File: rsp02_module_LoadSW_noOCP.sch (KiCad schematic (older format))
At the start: 9 parts, among them Q22 SISS23DN-T1-GE3, Q23 IRF7404, Q24 BC848B

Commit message: Update PCB
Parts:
- R90, R91, R92, R93: footprint Resistor_SMD:R_0402_1005Metric -> Resistor_SMD:R_0603_1608Metric
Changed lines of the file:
@@
 F 0 "R90" H 7000 1750 50  0000 L CNN
 F 1 "100k" H 7000 1550 50  0000 L CNN
-F 2 "Resistor_SMD:R_0402_1005Metric" V 6880 1650 50  0001 C CNN
+F 2 "Resistor_SMD:R_0603_1608Metric" V 6880 1650 50  0001 C CNN
 F 3 "~" H 6950 1650 50  0001 C CNN
 	1    6950 1650
@@
 F 0 "R93" H 9300 2250 50  0000 L CNN
 F 1 "100k" H 9300 2050 50  0000 L CNN
-F 2 "Resistor_SMD:R_0402_1005Metric" V 9180 2150 50  0001 C CNN
+F 2 "Resistor_SMD:R_0603_1608Metric" V 9180 2150 50  0001 C CNN
 F 3 "~" H 9250 2150 50  0001 C CNN
 	1    9250 2150
@@
 F 0 "R92" H 8850 5000 50  0000 L CNN
 F 1 "10k" H 8850 4800 50  0000 L CNN
-F 2 "Resistor_SMD:R_0402_1005Metric" V 8730 4900 50  0001 C CNN
+F 2 "Resistor_SMD:R_0603_1608Metric" V 8730 4900 50  0001 C CNN
 F 3 "~" H 8800 4900 50  0001 C CNN
 	1    8800 4900
@@
 F 0 "R91" V 8600 4550 50  0000 L CNN
 F 1 "10k" V 8400 4550 50  0000 L CNN
-F 2 "Resistor_SMD:R_0402_1005Metric" V 8430 4600 50  0001 C CNN
+F 2 "Resistor_SMD:R_0603_1608Metric" V 8430 4600 50  0001 C CNN
 F 3 "~" H 8500 4600 50  0001 C CNN
 	1    8500 4600

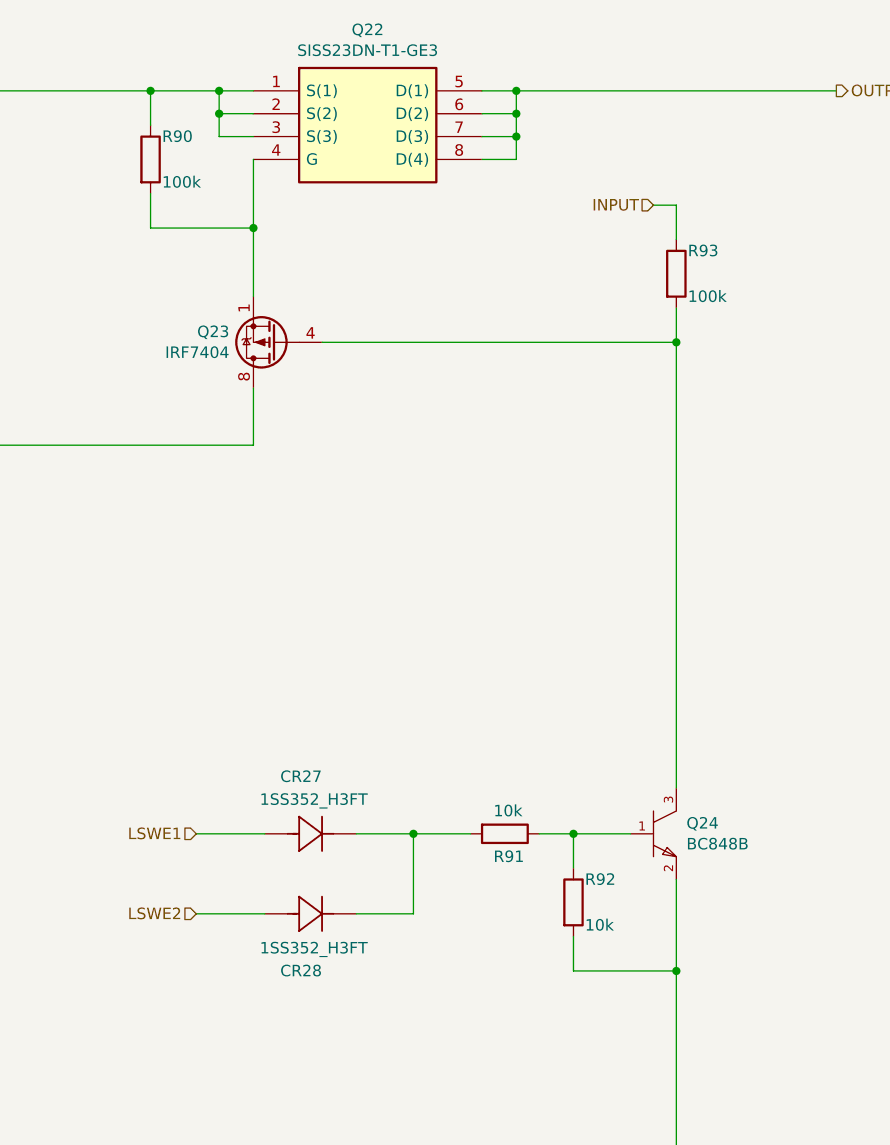
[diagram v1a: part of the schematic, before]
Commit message: PCB Update
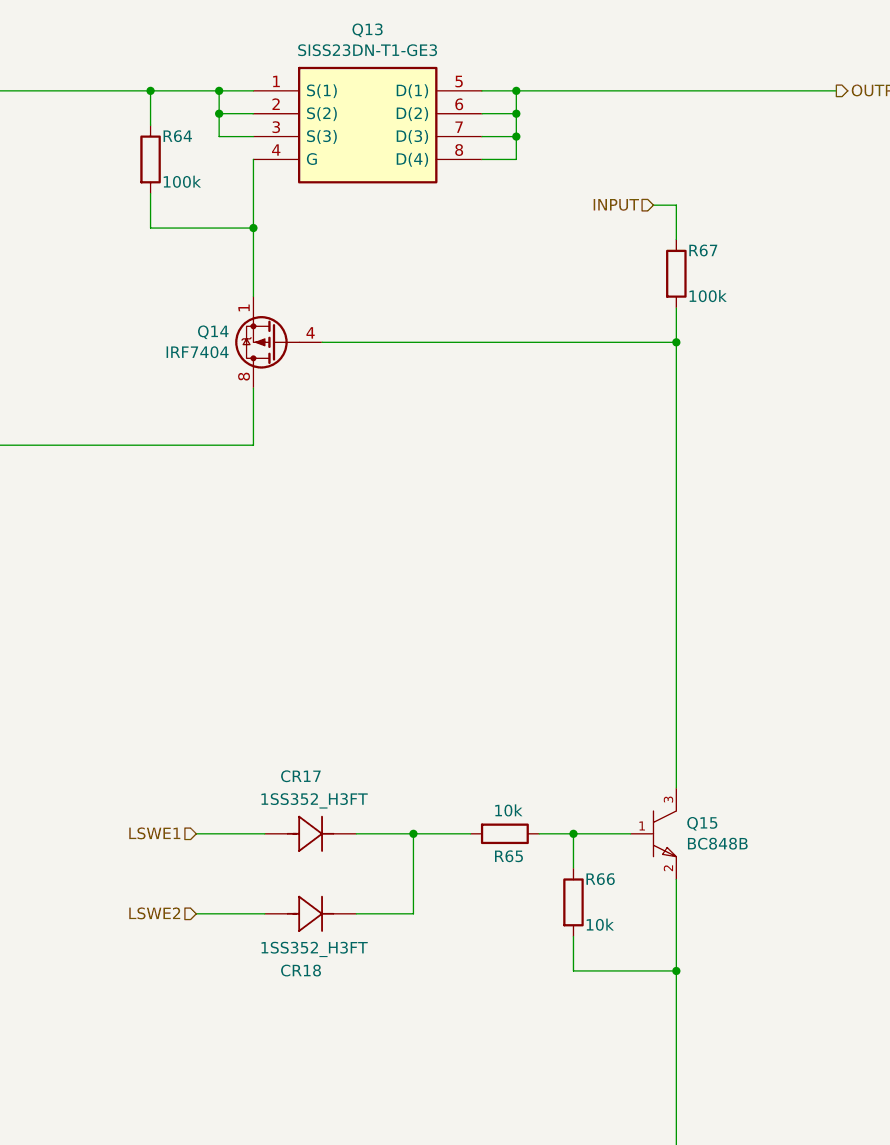
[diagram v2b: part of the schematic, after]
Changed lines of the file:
@@
 $Descr A4 11693 8268
 encoding utf-8
-Sheet 9 17
+Sheet 6 17
 Title "rsp02_module_LoadSW_OCP_noOCP"
 Date "2020-12-07"
@@
 AR Path="/5FD193EF/5FD0BC5C" Ref="Q22"  Part="1"
 AR Path="/5FD18D34/5FD0BC5C" Ref="Q13"  Part="1"
-F 0 "Q22" H 7900 1617 50  0000 C CNN
+F 0 "Q13" H 7900 1617 50  0000 C CNN
 F 1 "SISS23DN-T1-GE3" H 7900 1526 50  0000 C CNN
 F 2 "mypartsLib:POWERPAK-1212-8" H 7900 800 50  0001 C CNN
@@
 AR Path="/5FD193EF/5FD0BC5D" Ref="R90"  Part="1"
 AR Path="/5FD18D34/5FD0BC5D" Ref="R64"  Part="1"
-F 0 "R90" H 7000 1750 50  0000 L CNN
+F 0 "R64" H 7000 1750 50  0000 L CNN
 F 1 "100k" H 7000 1550 50  0000 L CNN
 F 2 "Resistor_SMD:R_0603_1608Metric" V 6880 1650 50  0001 C CNN
@@
 AR Path="/5FD193EF/5FD0BC5E" Ref="R93"  Part="1"
 AR Path="/5FD18D34/5FD0BC5E" Ref="R67"  Part="1"
-F 0 "R93" H 9300 2250 50  0000 L CNN
+F 0 "R67" H 9300 2250 50  0000 L CNN
 F 1 "100k" H 9300 2050 50  0000 L CNN
 F 2 "Resistor_SMD:R_0603_1608Metric" V 9180 2150 50  0001 C CNN
@@
 AR Path="/5FD193EF/5FD0BC5F" Ref="R92"  Part="1"
 AR Path="/5FD18D34/5FD0BC5F" Ref="R66"  Part="1"
-F 0 "R92" H 8850 5000 50  0000 L CNN
+F 0 "R66" H 8850 5000 50  0000 L CNN
 F 1 "10k" H 8850 4800 50  0000 L CNN
 F 2 "Resistor_SMD:R_0603_1608Metric" V 8730 4900 50  0001 C CNN
@@
 AR Path="/5FD193EF/5FD2B5CE" Ref="Q24"  Part="1"
 AR Path="/5FD18D34/5FD2B5CE" Ref="Q15"  Part="1"
-F 0 "Q24" H 9294 4646 50  0000 L CNN
+F 0 "Q15" H 9294 4646 50  0000 L CNN
 F 1 "BC848B" H 9294 4555 50  0000 L CNN
 F 2 "Package_TO_SOT_SMD:SOT-23" H 8950 5100 50  0001 L CNN
@@
 AR Path="/5FD193EF/5FD2B5CD" Ref="Q23"  Part="1"
 AR Path="/5FD18D34/5FD2B5CD" Ref="Q14"  Part="1"
-F 0 "Q23" H 7705 2404 50  0000 L CNN
+F 0 "Q14" H 7705 2404 50  0000 L CNN
 F 1 "IRF7404" H 7705 2495 50  0000 L CNN
 F 2 "Package_SO:SOIC-8_3.9x4.9mm_P1.27mm" H 7700 2375 50  0001 L CIN
@@
 AR Path="/5FD193EF/5FD2B5CF" Ref="CR28"  Part="1"
 AR Path="/5FD18D34/5FD2B5CF" Ref="CR18"  Part="1"
-F 0 "CR28" H 7700 4700 50  0000 R CNN
+F 0 "CR18" H 7700 4700 50  0000 R CNN
 F 1 "1SS352_H3FT" H 7900 4800 50  0000 R CNN
 F 2 "mypartsLib:1SS352_H3FT" H 7650 4700 60  0001 C CNN
@@
 AR Path="/5FD193EF/5FD2B5D0" Ref="CR27"  Part="1"
 AR Path="/5FD18D34/5FD2B5D0" Ref="CR17"  Part="1"
-F 0 "CR27" H 7700 4850 50  0000 R CNN
+F 0 "CR17" H 7700 4850 50  0000 R CNN
 F 1 "1SS352_H3FT" H 7900 4750 50  0000 R CNN
 F 2 "mypartsLib:1SS352_H3FT" H 7650 4350 60  0001 C CNN
@@
 AR Path="/5FD193EF/5FD0BC64" Ref="R91"  Part="1"
 AR Path="/5FD18D34/5FD0BC64" Ref="R65"  Part="1"
-F 0 "R91" V 8600 4550 50  0000 L CNN
+F 0 "R65" V 8600 4550 50  0000 L CNN
 F 1 "10k" V 8400 4550 50  0000 L CNN
 F 2 "Resistor_SMD:R_0603_1608Metric" V 8430 4600 50  0001 C CNN

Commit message: PCB Design Finished
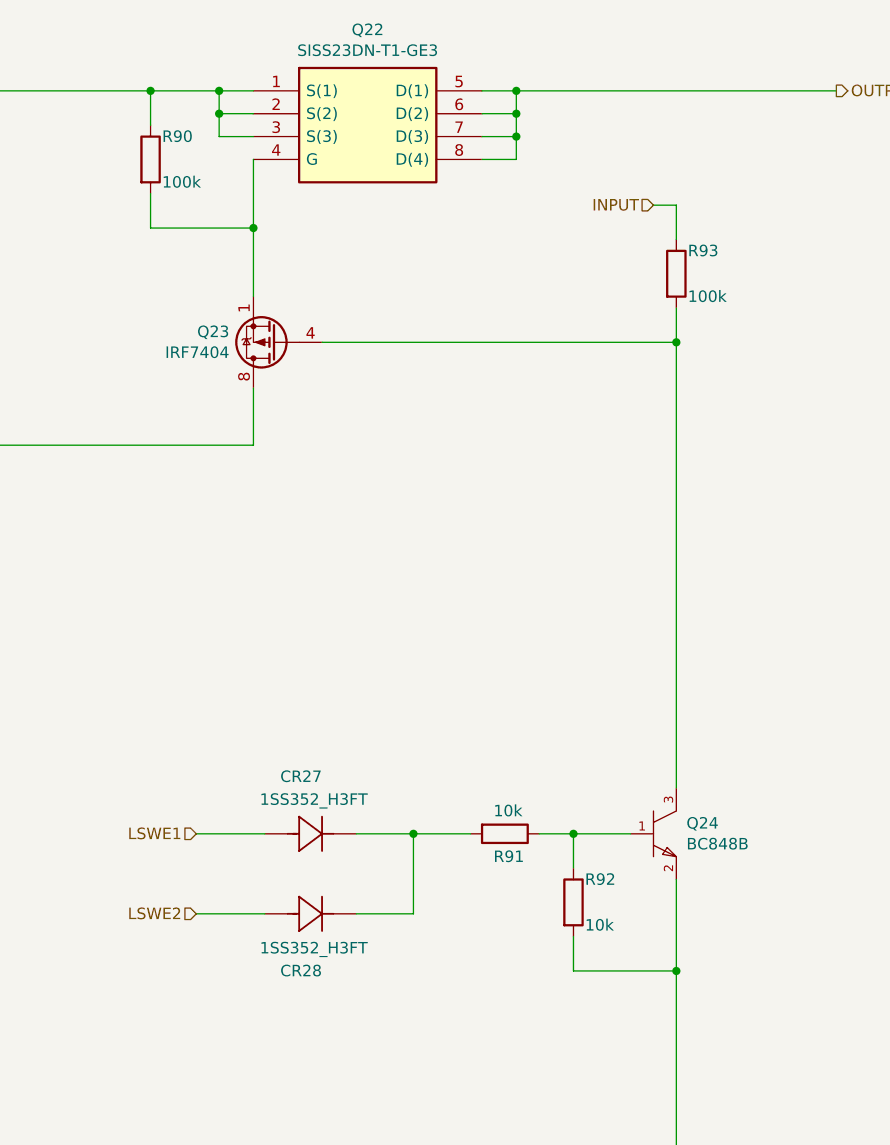
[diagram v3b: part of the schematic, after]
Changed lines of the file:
@@
 $Descr A4 11693 8268
 encoding utf-8
-Sheet 6 17
+Sheet 9 17
 Title "rsp02_module_LoadSW_OCP_noOCP"
 Date "2020-12-07"
@@
 AR Path="/5FD193EF/5FD0BC5C" Ref="Q22"  Part="1"
 AR Path="/5FD18D34/5FD0BC5C" Ref="Q13"  Part="1"
-F 0 "Q13" H 7900 1617 50  0000 C CNN
+F 0 "Q22" H 7900 1617 50  0000 C CNN
 F 1 "SISS23DN-T1-GE3" H 7900 1526 50  0000 C CNN
 F 2 "mypartsLib:POWERPAK-1212-8" H 7900 800 50  0001 C CNN
@@
 AR Path="/5FD193EF/5FD0BC5D" Ref="R90"  Part="1"
 AR Path="/5FD18D34/5FD0BC5D" Ref="R64"  Part="1"
-F 0 "R64" H 7000 1750 50  0000 L CNN
+F 0 "R90" H 7000 1750 50  0000 L CNN
 F 1 "100k" H 7000 1550 50  0000 L CNN
 F 2 "Resistor_SMD:R_0603_1608Metric" V 6880 1650 50  0001 C CNN
@@
 AR Path="/5FD193EF/5FD0BC5E" Ref="R93"  Part="1"
 AR Path="/5FD18D34/5FD0BC5E" Ref="R67"  Part="1"
-F 0 "R67" H 9300 2250 50  0000 L CNN
+F 0 "R93" H 9300 2250 50  0000 L CNN
 F 1 "100k" H 9300 2050 50  0000 L CNN
 F 2 "Resistor_SMD:R_0603_1608Metric" V 9180 2150 50  0001 C CNN
@@
 AR Path="/5FD193EF/5FD0BC5F" Ref="R92"  Part="1"
 AR Path="/5FD18D34/5FD0BC5F" Ref="R66"  Part="1"
-F 0 "R66" H 8850 5000 50  0000 L CNN
+F 0 "R92" H 8850 5000 50  0000 L CNN
 F 1 "10k" H 8850 4800 50  0000 L CNN
 F 2 "Resistor_SMD:R_0603_1608Metric" V 8730 4900 50  0001 C CNN
@@
 AR Path="/5FD193EF/5FD2B5CE" Ref="Q24"  Part="1"
 AR Path="/5FD18D34/5FD2B5CE" Ref="Q15"  Part="1"
-F 0 "Q15" H 9294 4646 50  0000 L CNN
+F 0 "Q24" H 9294 4646 50  0000 L CNN
 F 1 "BC848B" H 9294 4555 50  0000 L CNN
 F 2 "Package_TO_SOT_SMD:SOT-23" H 8950 5100 50  0001 L CNN
@@
 AR Path="/5FD193EF/5FD2B5CD" Ref="Q23"  Part="1"
 AR Path="/5FD18D34/5FD2B5CD" Ref="Q14"  Part="1"
-F 0 "Q14" H 7705 2404 50  0000 L CNN
+F 0 "Q23" H 7705 2404 50  0000 L CNN
 F 1 "IRF7404" H 7705 2495 50  0000 L CNN
 F 2 "Package_SO:SOIC-8_3.9x4.9mm_P1.27mm" H 7700 2375 50  0001 L CIN
@@
 AR Path="/5FD193EF/5FD2B5CF" Ref="CR28"  Part="1"
 AR Path="/5FD18D34/5FD2B5CF" Ref="CR18"  Part="1"
-F 0 "CR18" H 7700 4700 50  0000 R CNN
+F 0 "CR28" H 7700 4700 50  0000 R CNN
 F 1 "1SS352_H3FT" H 7900 4800 50  0000 R CNN
 F 2 "mypartsLib:1SS352_H3FT" H 7650 4700 60  0001 C CNN
@@
 AR Path="/5FD193EF/5FD2B5D0" Ref="CR27"  Part="1"
 AR Path="/5FD18D34/5FD2B5D0" Ref="CR17"  Part="1"
-F 0 "CR17" H 7700 4850 50  0000 R CNN
+F 0 "CR27" H 7700 4850 50  0000 R CNN
 F 1 "1SS352_H3FT" H 7900 4750 50  0000 R CNN
 F 2 "mypartsLib:1SS352_H3FT" H 7650 4350 60  0001 C CNN
@@
 AR Path="/5FD193EF/5FD0BC64" Ref="R91"  Part="1"
 AR Path="/5FD18D34/5FD0BC64" Ref="R65"  Part="1"
-F 0 "R65" V 8600 4550 50  0000 L CNN
+F 0 "R91" V 8600 4550 50  0000 L CNN
 F 1 "10k" V 8400 4550 50  0000 L CNN
 F 2 "Resistor_SMD:R_0603_1608Metric" V 8430 4600 50  0001 C CNN
